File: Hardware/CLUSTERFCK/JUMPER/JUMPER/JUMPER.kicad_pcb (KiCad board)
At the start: 2 copper layers, 142 x 52.3 mm, 3 parts, among them J1 Conn_02x20_Counter_Clockwise, J2 Conn_02x20_Counter_Clockwise

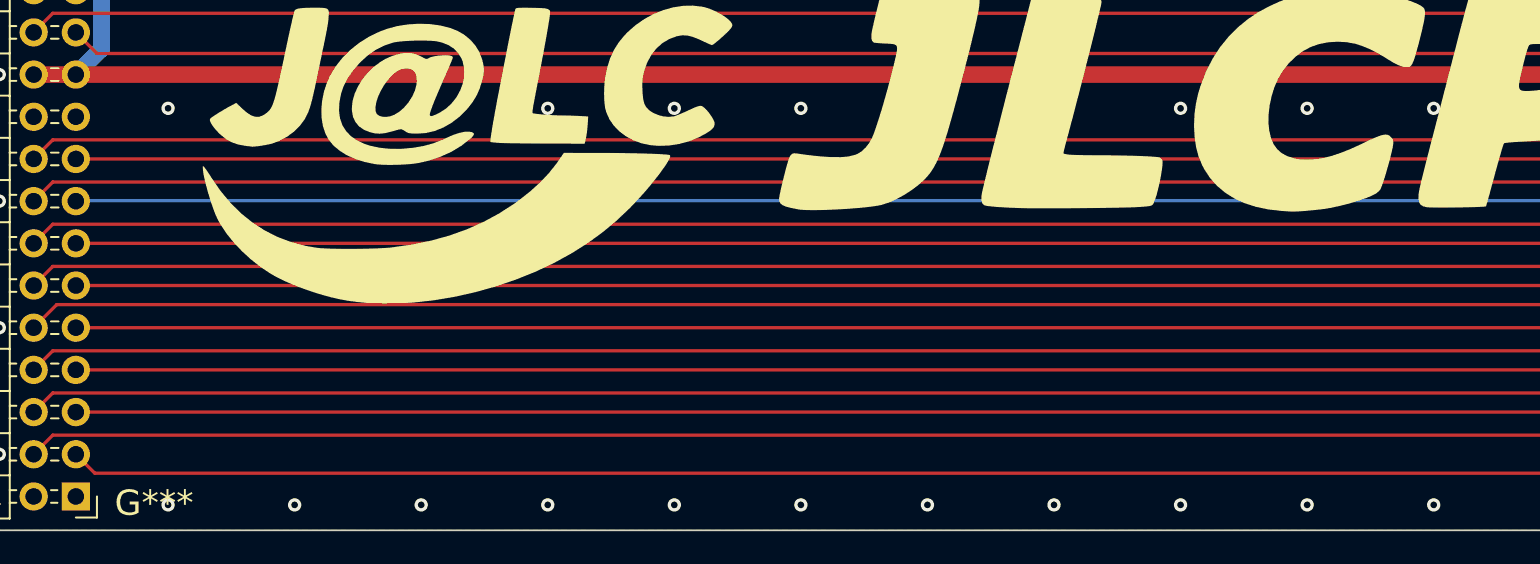
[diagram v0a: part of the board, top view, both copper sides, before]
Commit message: 0072 | 3h | make silkscreen prettier
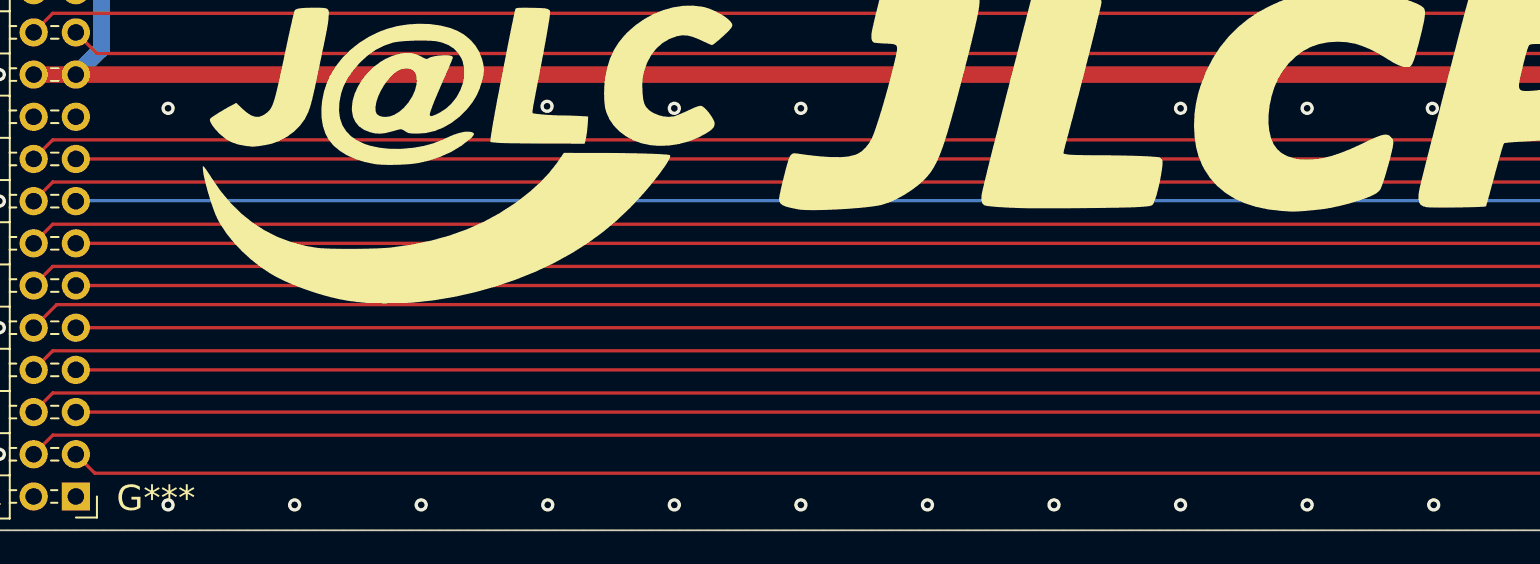
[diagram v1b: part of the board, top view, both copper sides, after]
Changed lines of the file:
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@@
     (at 71.8 26.9)
     (attr through_hole)
-    (fp_text reference "G***" (at -60.45 23.8) (layer "F.SilkS")
+    (fp_text reference "G***" (at -60.34 23.51) (layer "F.SilkS")
       (effects (font (size 1.524 1.524) (thickness 0.3)))
     )
@@
   (via (at 111.252 26.932) (size 0.8) (drill 0.4) (layers "F.Cu" "B.Cu") (free) (net 9))
   (via (at 65.532 12.2) (size 0.8) (drill 0.4) (layers "F.Cu" "B.Cu") (free) (net 9))
-  (via (at 35.052 26.932) (size 0.8) (drill 0.4) (layers "F.Cu" "B.Cu") (free) (net 9))
+  (via (at 35.01 26.81) (size 0.8) (drill 0.4) (layers "F.Cu" "B.Cu") (free) (net 9))
   (via (at 65.532 26.932) (size 0.8) (drill 0.4) (layers "F.Cu" "B.Cu") (free) (net 9))
   (via (at 126.492 50.808) (size 0.8) (drill 0.4) (layers "F.Cu" "B.Cu") (free) (net 9))
@@
   (via (at 27.432 12.2) (size 0.8) (drill 0.4) (layers "F.Cu" "B.Cu") (free) (net 9))
   (via (at 57.912 50.808) (size 0.8) (drill 0.4) (layers "F.Cu" "B.Cu") (free) (net 9))
-  (via (at 88.392 26.932) (size 0.8) (drill 0.4) (layers "F.Cu" "B.Cu") (free) (net 9))
+  (via (at 88.31 26.932) (size 0.8) (drill 0.4) (layers "F.Cu" "B.Cu") (free) (net 9))
   (via (at 19.812 12.2) (size 0.8) (drill 0.4) (layers "F.Cu" "B.Cu") (free) (net 9))
   (via (at 2.032 2.04) (size 0.8) (drill 0.4) (layers "F.Cu" "B.Cu") (free) (net 9))
